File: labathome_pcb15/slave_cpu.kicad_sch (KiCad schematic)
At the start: 45 parts, among them J1 HALL, J25 TC-2030, J26 PROG STM, J27 ADDA, J28 Brushless, J34 STM32 EXT, U16 LM358, U3 DRV8313, U5 STM32G431R8Tx

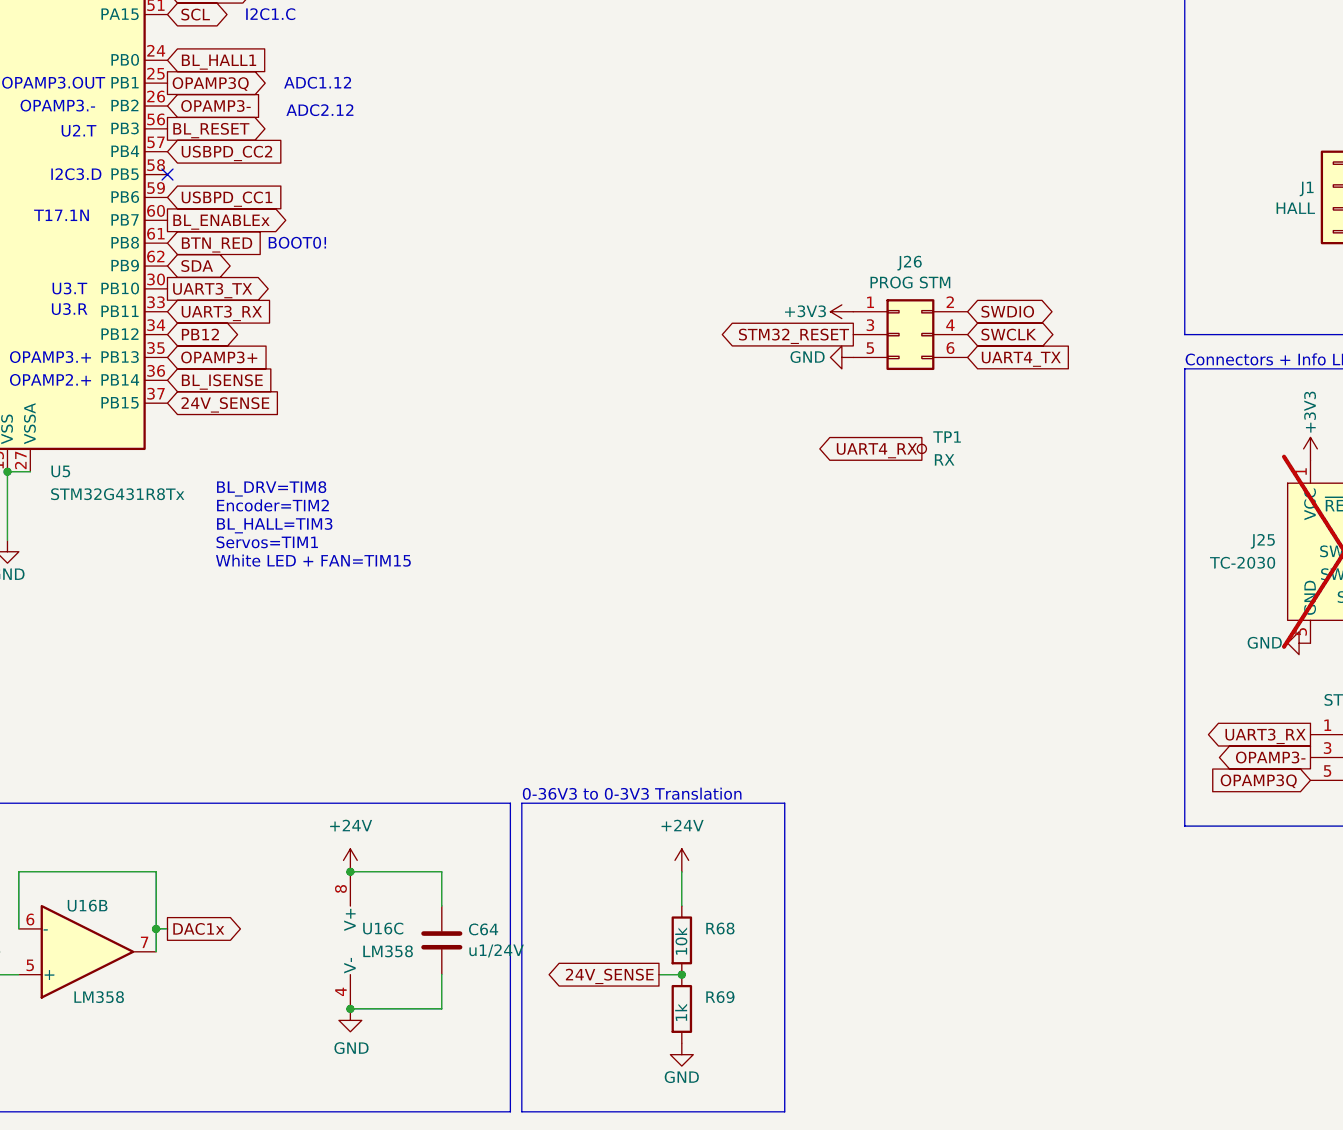
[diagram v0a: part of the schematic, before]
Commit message: Minimal changes
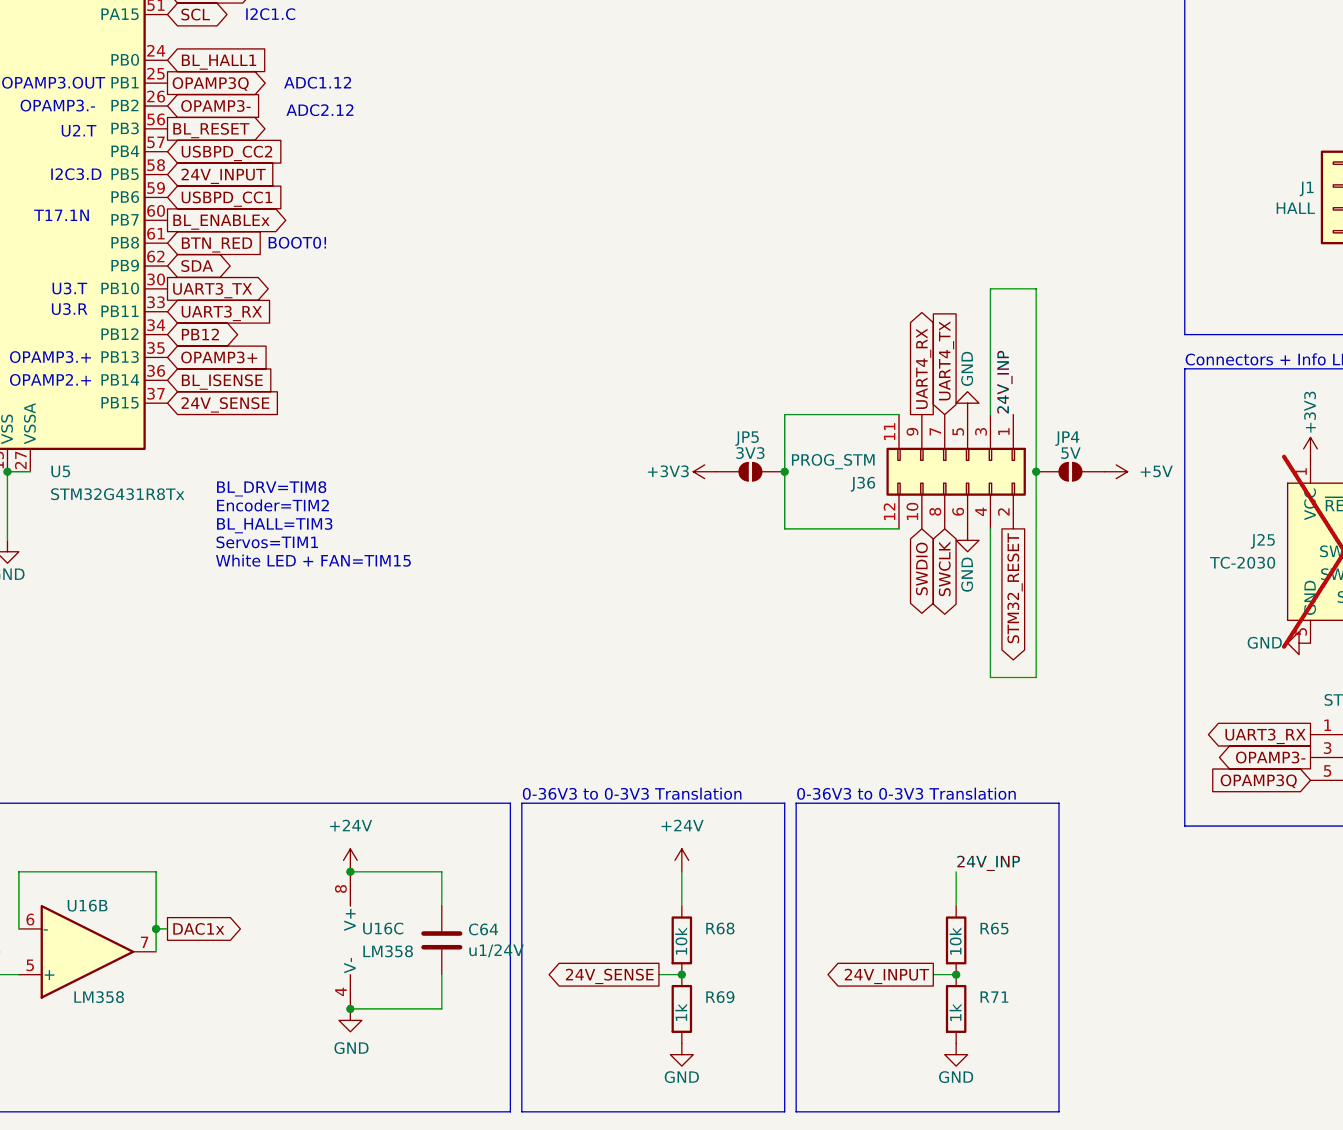
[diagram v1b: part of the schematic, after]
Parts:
- removed J26: PROG STM, liebler_CONN:PinHeader_2x03_P1.27mm_Vertical_SMD_handsolder, symbol Connector_Generic:Conn_02x03_Odd_Even
- removed TP1: RX, TestPoint:TestPoint_THTPad_D1.5mm_Drill0.7mm, symbol Connector:TestPoint_Small
- added J36: PROG_STM, Connector_PinSocket_2.54mm:PinSocket_2x06_P2.54mm_Vertical_SMD, symbol Connector_Generic:Conn_02x06_Odd_Even
- added JP4: 5V, Jumper:SolderJumper-2_P1.3mm_Open_RoundedPad1.0x1.5mm, symbol Jumper:SolderJumper_2_Open
- added JP5: 3V3, Jumper:SolderJumper-2_P1.3mm_Open_RoundedPad1.0x1.5mm, symbol Jumper:SolderJumper_2_Open
- added R65: 10k, Resistor_SMD:R_0201_0603Metric, symbol Device:R
- added R71: 1k, Resistor_SMD:R_0402_1005Metric, symbol Device:R
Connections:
- net +3V3: now also JP5.1 (A)
- net GND: now also J36.5 (Pin_5), J36.6 (Pin_6), R71.2
- net STM32_RESET: now also J36.2 (Pin_2)
- net SWCLK: now also J36.8 (Pin_8)
- net SWDIO: now also J36.10 (Pin_10)
- net UART4_RX: now also J36.9 (Pin_9)
- net UART4_TX: now also J36.7 (Pin_7)
- net 24V_INPUT: now reaches U5.58 (PB5)
- net 24V_INPUT: now also R65.2, R71.1
- new net: J36.11 (Pin_11), J36.12 (Pin_12), JP5.2 (B)
- new net: J36.3 (Pin_3), J36.4 (Pin_4), JP4.1 (A)
- new net +5V: JP4.2 (B)
- new net 24V_INP: J36.1 (Pin_1), R65.1
- no-connect marks 2 -> 1

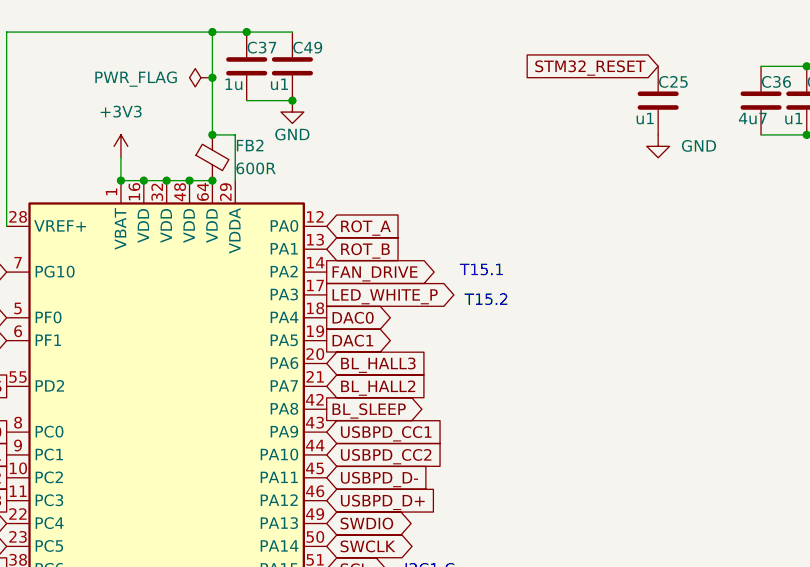
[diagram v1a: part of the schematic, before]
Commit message: IP5306
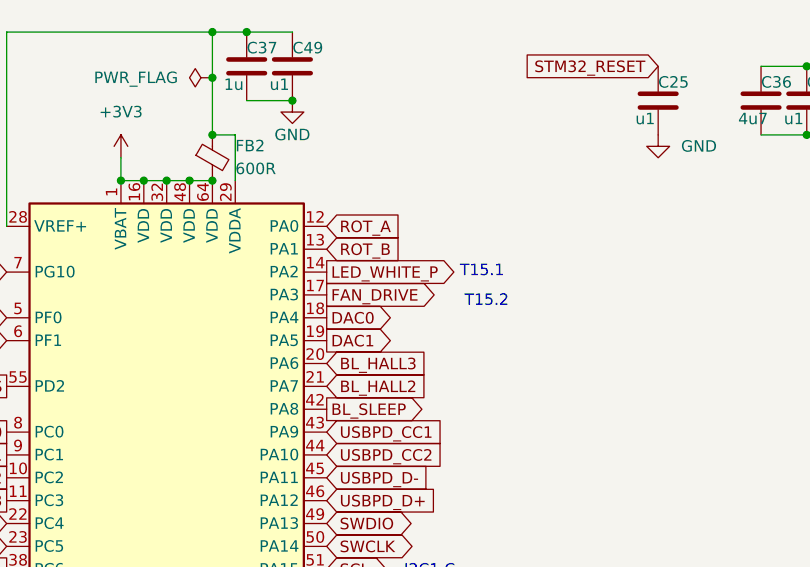
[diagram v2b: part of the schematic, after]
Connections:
- net FAN_DRIVE: now also U5.17 (PA3); no longer U5.14 (PA2)
- net LED_WHITE_P: now also U5.14 (PA2); no longer U5.17 (PA3)
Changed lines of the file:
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@@
 	(global_label "FAN_DRIVE"
 		(shape output)
-		(at 68.58 41.91 0)
+		(at 68.58 44.45 0)
 		(fields_autoplaced yes)
 		(effects
@@
 		)
 		(property "Intersheetrefs" "${INTERSHEET_REFS}"
-			(at 81.4229 41.91 0)
+			(at 81.4229 44.45 0)
 			(effects
 				(font
@@
 	(global_label "LED_WHITE_P"
 		(shape output)
-		(at 68.58 44.45 0)
+		(at 68.58 41.91 0)
 		(fields_autoplaced yes)
 		(effects
@@
 		)
 		(property "Intersheetrefs" "${INTERSHEET_REFS}"
-			(at 83.7208 44.45 0)
+			(at 83.7208 41.91 0)
 			(effects
 				(font

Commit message: bsec
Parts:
- C39: footprint Capacitor_THT:CP_Radial_D6.3mm_P2.50mm -> Capacitor_SMD:CP_Elec_6.3x5.4
- R38: footprint Resistor_THT:R_Axial_DIN0309_L9.0mm_D3.2mm_P12.70mm_Horizontal -> Resistor_SMD:R_2512_6332Metric
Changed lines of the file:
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@@
 			)
 		)
-		(property "Footprint" "Resistor_THT:R_Axial_DIN0309_L9.0mm_D3.2mm_P12.70mm_Horizontal"
+		(property "Footprint" "Resistor_SMD:R_2512_6332Metric"
 			(at 248.412 59.69 90)
 			(effects
@@
 			)
 		)
-		(property "Footprint" "Capacitor_THT:CP_Radial_D6.3mm_P2.50mm"
+		(property "Footprint" "Capacitor_SMD:CP_Elec_6.3x5.4"
 			(at 263.8552 66.04 0)
 			(effects
